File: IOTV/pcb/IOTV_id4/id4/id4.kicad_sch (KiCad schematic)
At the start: 7 parts, among them J1 Conn_01x04, J2 Conn_01x03, U1 WeMos_D1_mini

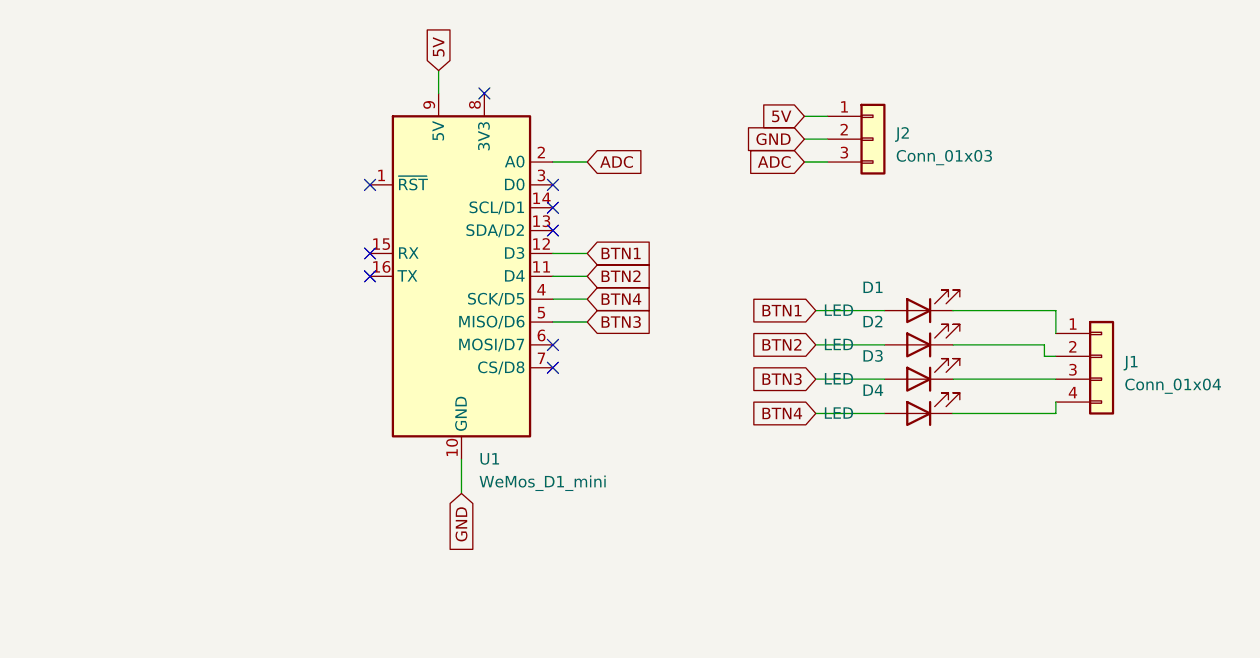
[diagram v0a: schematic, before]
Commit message: pcb id4
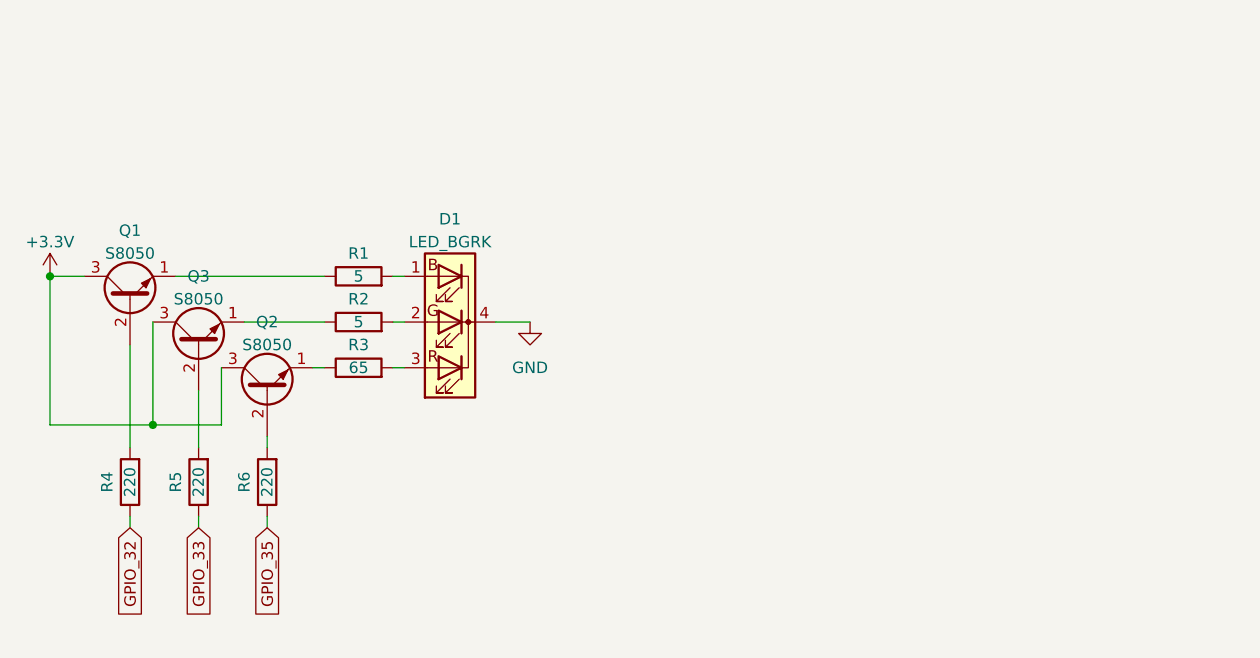
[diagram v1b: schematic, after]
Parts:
- removed D1, D2, D3, D4: LED, LED_THT:LED_D2.0mm_W4.8mm_H2.5mm_FlatTop, symbol Device:LED
- removed J1: Conn_01x04, Jumper:tht_jumper_x4-2.54mm, symbol PCM_4ms_Connector:Conn_01x04
- removed J2: Conn_01x03, Jumper:tht_jumper_x3-2.54mm, symbol PCM_4ms_Connector:Conn_01x03
- removed U1: WeMos_D1_mini, Module:WEMOS_D1_mini_light, symbol MCU_Module:WeMos_D1_mini
- added D1: LED_BGRK, symbol Device:LED_BGRK
- added Q1, Q2, Q3: S8050, Package_TO_SOT_THT:TO-92_Inline, symbol Transistor_BJT:S8050
- added R1, R2: 5, symbol Device:R
- added R3: 65, symbol Device:R
- added R4, R5, R6: 220, symbol Device:R
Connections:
- net GND: now also D1.4 (K)
- new net: Q1.2 (B), R4.2
- new net: Q1.1 (E), R1.1
- new net: D1.1 (BA), R1.2
- new net: Q3.1 (E), R2.1
- new net: D1.2 (GA), R2.2
- new net: Q3.2 (B), R5.2
- new net: Q2.1 (E), R3.1
- new net: D1.3 (RA), R3.2
- new net: Q2.2 (B), R6.2
- new net +3.3V: Q1.3 (C), Q2.3 (C), Q3.3 (C)
- new net GPIO_32: R4.1
- new net GPIO_33: R5.1
- new net GPIO_35: R6.1
- no-connect marks 9 -> 0
